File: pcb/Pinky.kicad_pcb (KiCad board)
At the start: 2 copper layers, 142.2 x 120.5 mm, 78 parts, among them J1 MJ-4PP-9, P1 i2c-pin, P2 i2c-pin, SW1 RESET_SW, SW10 SW_PUSH, SW11 SW_PUSH, SW12 SW_PUSH, SW13 SW_PUSH, SW14 SW_PUSH, SW15 SW_PUSH, SW16 SW_PUSH, SW17 SW_PUSH, SW18 SW_PUSH, SW19 SW_PUSH, SW2 SW_PUSH, SW20 SW_PUSH, SW21 SW_PUSH, SW22 SW_PUSH, SW23 SW_PUSH, SW24 SW_PUSH, SW25 SW_PUSH, SW26 SW_PUSH, SW27 SW_PUSH, SW28 SW_PUSH, SW29 SW_PUSH, SW3 SW_PUSH, SW30 SW_PUSH, SW31 SW_PUSH, SW32 SW_PUSH, SW33 SW_PUSH, SW4 SW_PUSH, SW5 SW_PUSH, SW6 SW_PUSH, SW7 SW_PUSH, SW8 SW_PUSH, SW9 SW_PUSH, U1 ProMicro

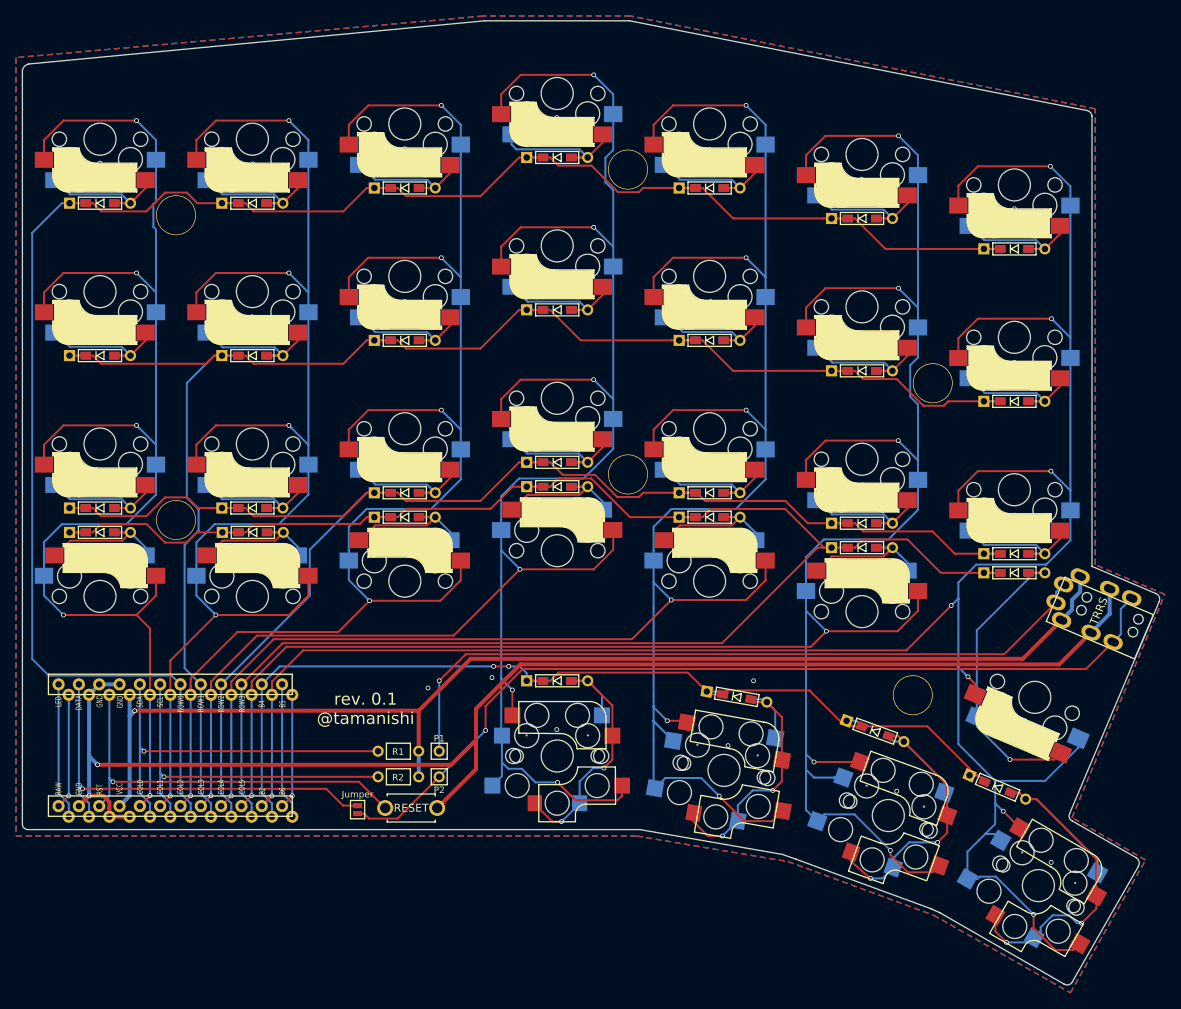
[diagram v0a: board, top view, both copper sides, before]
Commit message: sent to allpcb
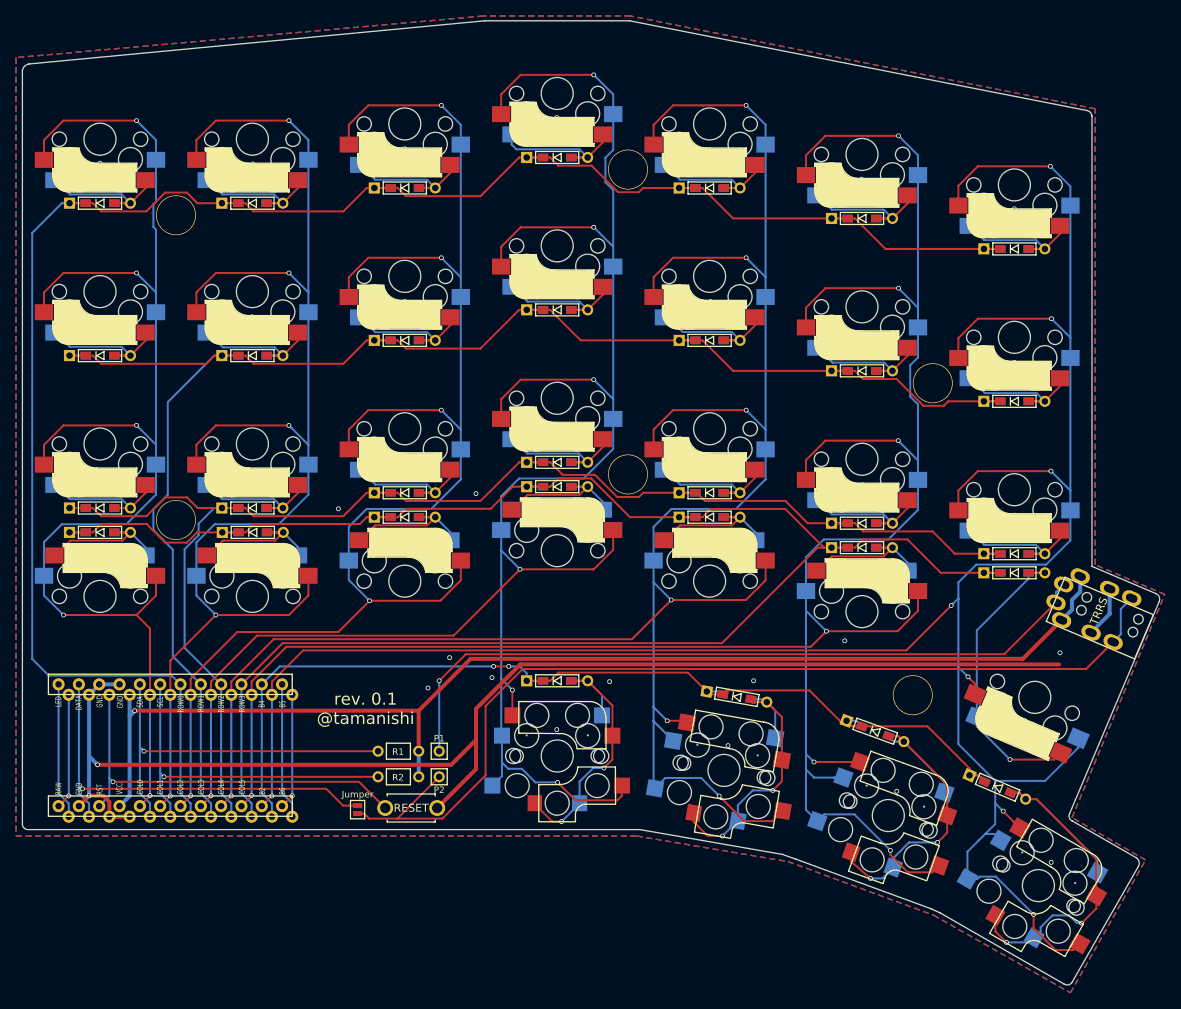
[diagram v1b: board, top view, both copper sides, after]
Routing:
- net Net-(J1-PadB): track 112.1 -> 122.7 mm, vias 1 -> 0
- net row2: track 191.6 -> 185.5 mm
- net GND: track 178.1 -> 172.4 mm, vias 29 -> 35
- net row1: track 203.6 -> 205.7 mm
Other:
- rule pad_to_mask_clearance: 0.051 -> 0.2
